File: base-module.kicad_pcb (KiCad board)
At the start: 4 copper layers, 100 x 100 mm, 147 parts, among them J200 09031967921, J800 USB_C_Receptacle_USB2.0_16P, Q700 MMST3904, SW400 TL2243, U100 W25Q128, U200 IP4234CZ6,115, U300 TPS563201DDCR, U301 TPS563201DDCR, U302 CH334P, U400 STM32H750VBTx, U500 TJA1044GTK_3Z, U600 TJA1044GTK_3Z, U700 STM32F103CBTx, U800 IP4234CZ6,115, U801 FSUSB42UMX, X300 Q13FC1350000400, X400 X322512MSB4SI, Y700 8 MHz, Y900 12Mhz

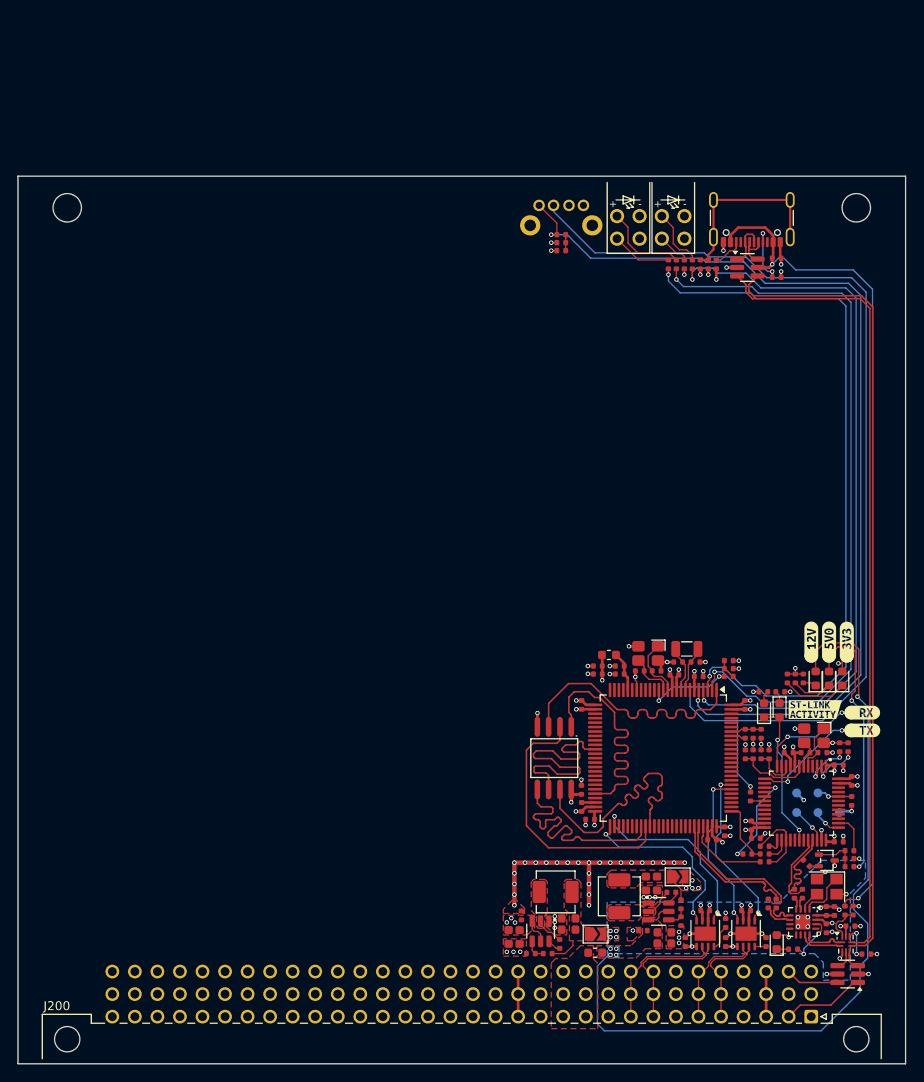
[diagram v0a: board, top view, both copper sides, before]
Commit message: [#2] Add grid and drill origin
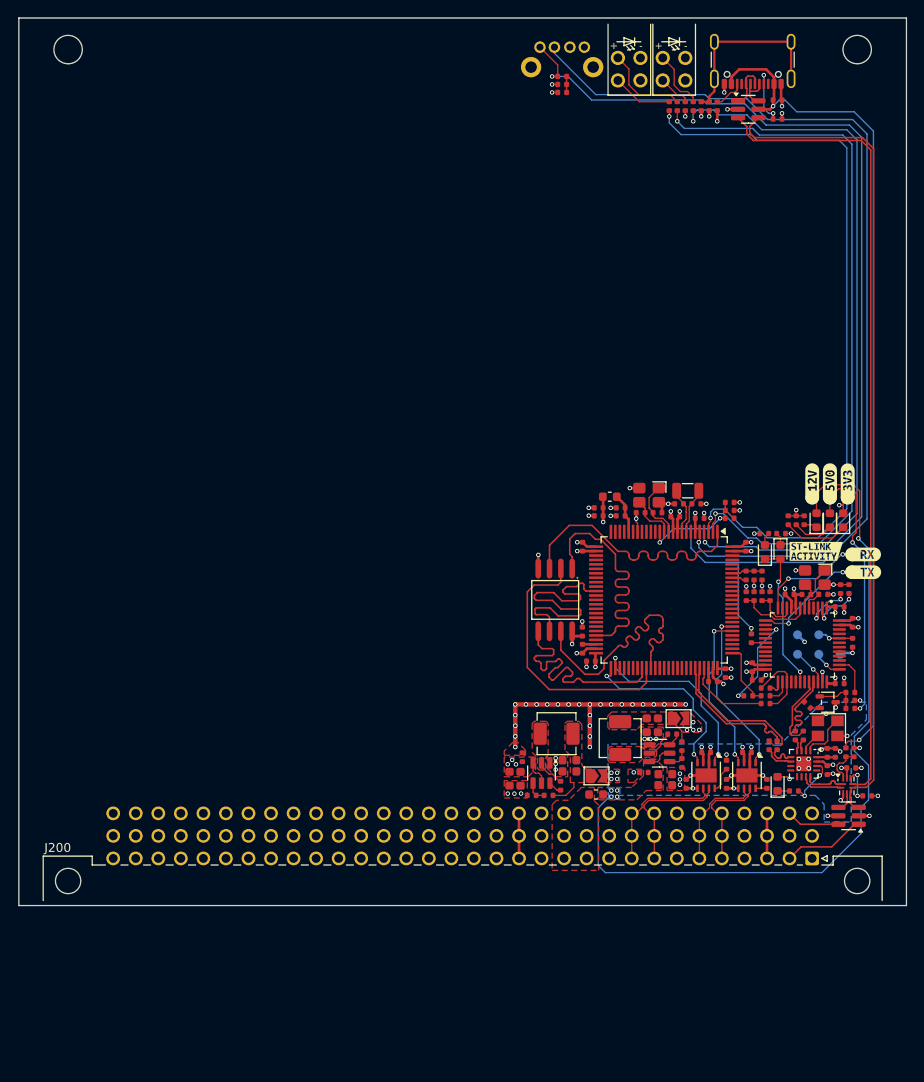
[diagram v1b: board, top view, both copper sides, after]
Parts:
- moved C301 17.8 mm to (101.4, 136.2)
- moved C302 17.8 mm to (101.4, 134.9)
- moved C305 17.8 mm to (96.1, 134.6)
- moved C309 17.8 mm to (112.2, 137.7)
- moved C310 17.8 mm to (112.2, 136.5)
- moved C402 17.8 mm to (102.9, 110.8)
- moved C404 17.8 mm to (119.0, 125.1)
- moved C405 17.8 mm to (121.3, 110.8)
- moved C410 17.8 mm to (123.1, 114.1)
- moved C413 17.8 mm to (102.9, 122.3)
- moved C501 17.8 mm to (119.1, 137.6)
- moved C601 17.8 mm to (114.5, 137.6)
- moved C707 17.8 mm to (130.0, 116.2)
- moved C900 17.8 mm to (130.4, 134.1)
- moved C902 17.8 mm to (131.3, 134.1)
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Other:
- outline, holes or cut-outs redrawn
